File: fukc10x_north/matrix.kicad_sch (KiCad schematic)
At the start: 237 parts

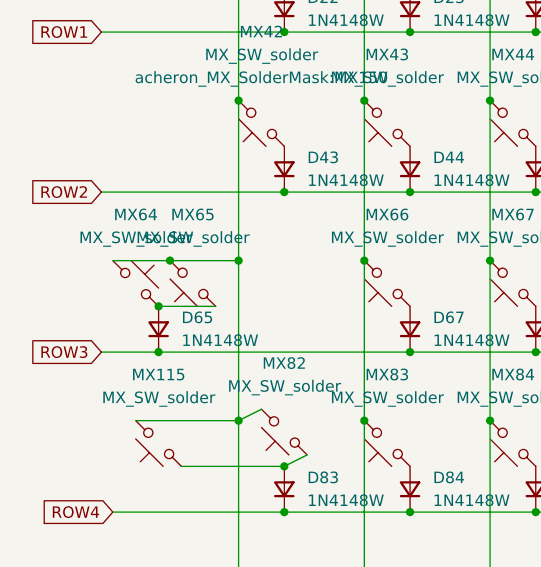
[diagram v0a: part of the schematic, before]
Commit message: fixed some shenanaigans
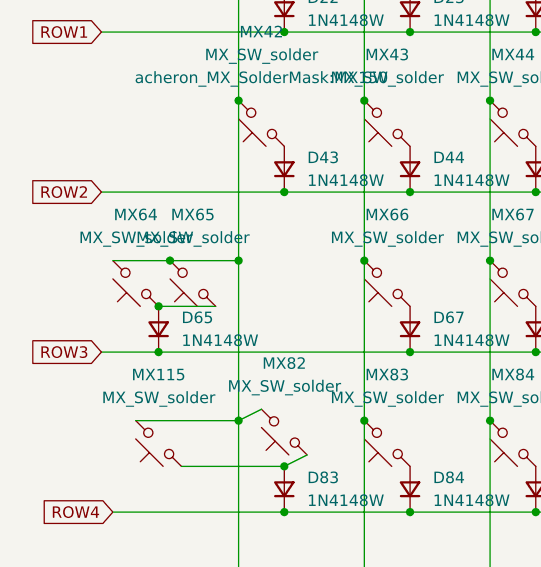
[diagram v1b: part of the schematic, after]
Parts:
- MX110: footprint acheron_MX_SolderMask:MX100 -> acheron_MX_SolderMask:MX200R
- MX77: footprint acheron_MX_SolderMask:MX250R -> acheron_MX_SolderMask:MX225R
- MX82: footprint acheron_MX_SolderMask:MX250 -> acheron_MX_SolderMask:MX225
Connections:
- net COL0: now also MX64.2; no longer MX64.1
- net at D65.2 (A), MX65.1: now also MX64.1; no longer MX64.2
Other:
- moved on the sheet: MX64
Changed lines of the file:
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@@
 	)
 	(junction
+		(at 27.94 95.25)
+		(diameter 0)
+		(color 0 0 0 0)
+	)
+	(junction
 		(at 97.79 64.77)
 		(diameter 0)
@@
 	)
 	(junction
-		(at 27.94 95.25)
-		(diameter 0)
-		(color 0 0 0 0)
-	)
-	(junction
 		(at 27.94 100.33)
 		(diameter 0)
@@
 	(symbol
 		(lib_id "PCM_marbastlib-mx:MX_SW_solder")
-		(at 25.4 92.71 0)
+		(at 25.4 92.71 180)
 		(unit 1)
 		(body_style 1)
@@
 			)
 		)
-		(property "Footprint" "acheron_MX_SolderMask:MX100"
+		(property "Footprint" "acheron_MX_SolderMask:MX200R"
 			(at 297.18 128.27 0)
 			(hide yes)
@@
 			)
 		)
-		(property "Footprint" "acheron_MX_SolderMask:MX250R"
+		(property "Footprint" "acheron_MX_SolderMask:MX225R"
 			(at 214.63 92.71 0)
 			(hide yes)
@@
 			)
 		)
-		(property "Footprint" "acheron_MX_SolderMask:MX250"
+		(property "Footprint" "acheron_MX_SolderMask:MX225"
 			(at 41.91 109.22 0)
 			(hide yes)
